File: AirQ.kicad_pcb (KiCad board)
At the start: 2 copper layers, 4 parts, among them U1 ESP32-H2-MINI-1-H2, U2 AP2112K-3.3, U3 AP2112K-1.8

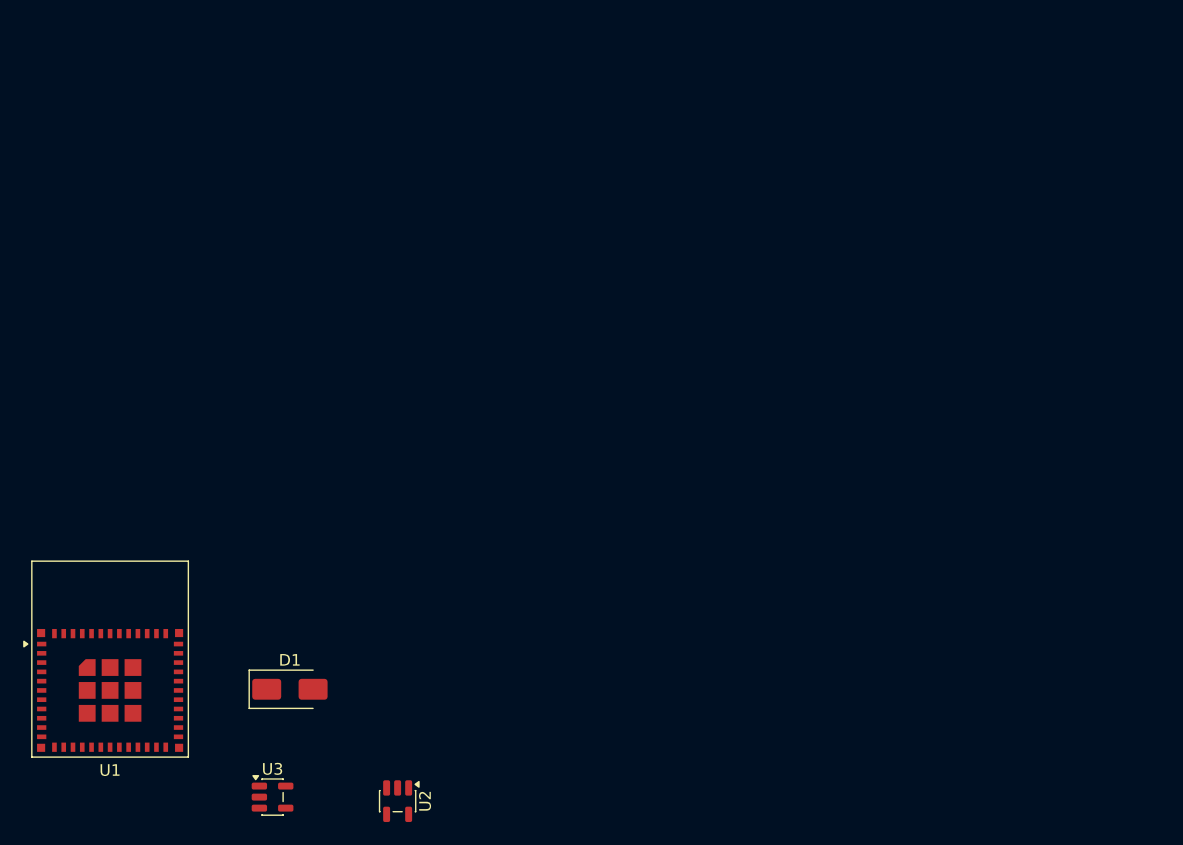
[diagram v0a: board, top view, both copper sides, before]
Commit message: Avances Viernes
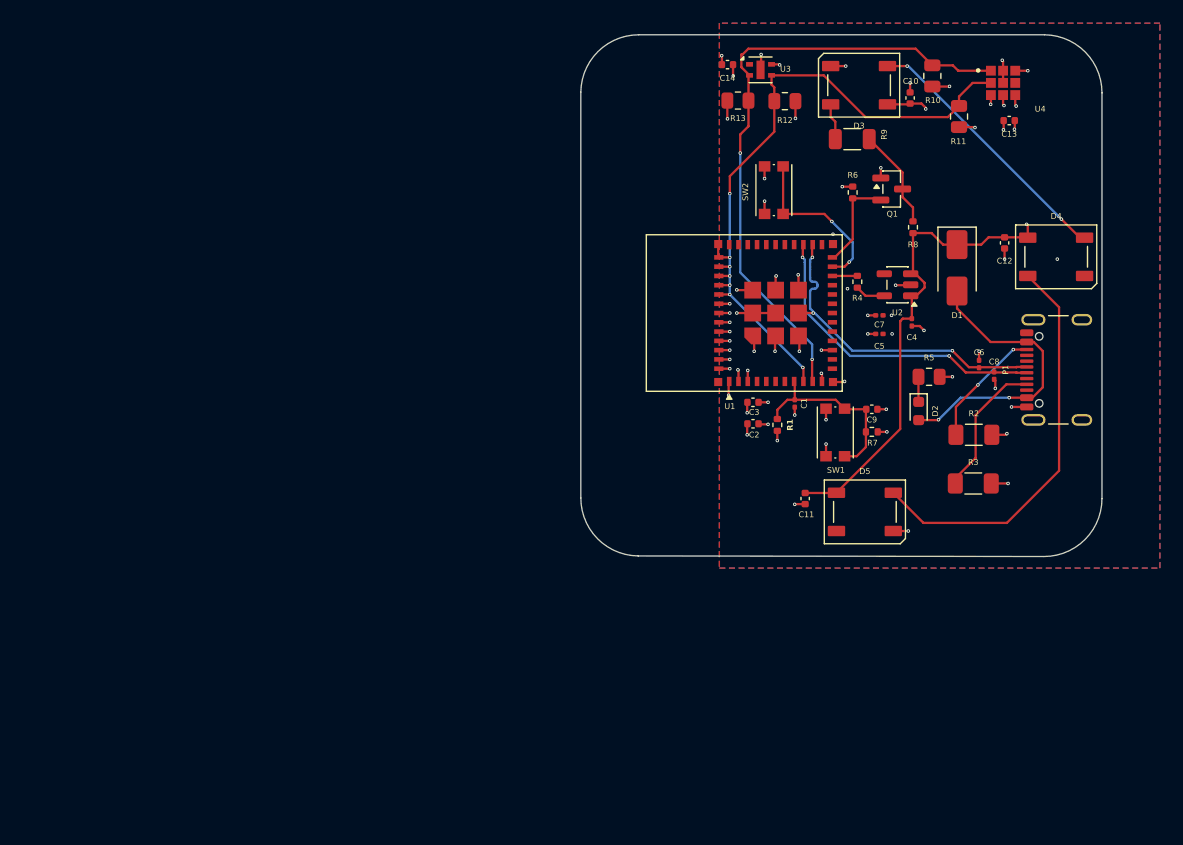
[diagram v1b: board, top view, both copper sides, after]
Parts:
- added C1: 1uF, Capacitor_SMD:C_0201_0603Metric, F.Cu at (173.5, 81.8)
- added C10: 0.1uF, Capacitor_SMD:C_0402_1005Metric, F.Cu at (183.4, 55.5)
- added C11: 0.1uF, Capacitor_SMD:C_0402_1005Metric, F.Cu at (174.4, 90.0)
- added C12: 0.1uF, Capacitor_SMD:C_0402_1005Metric, F.Cu at (191.6, 68.0)
- added C13: 10uF, Capacitor_SMD:C_0402_1005Metric, F.Cu at (192.0, 57.4)
- added C14: 0.1uF, Capacitor_SMD:C_0402_1005Metric, F.Cu at (167.7, 52.6)
- added C2: 10uF, Capacitor_SMD:C_0402_1005Metric, F.Cu at (169.9, 83.5)
- added C3: 0.1uF, Capacitor_SMD:C_0402_1005Metric, F.Cu at (169.9, 81.7)
- added C4: 1uF, Capacitor_SMD:C_0201_0603Metric, F.Cu at (183.6, 74.8)
- added C5: 1uF, Capacitor_SMD:C_0201_0603Metric, F.Cu at (180.8, 75.8)
- added C6: 1uF, Capacitor_SMD:C_0201_0603Metric, F.Cu at (189.4, 78.4)
- added C7: 1uF, Capacitor_SMD:C_0201_0603Metric, F.Cu at (180.8, 74.2)
- added C8: 1uF, Capacitor_SMD:C_0201_0603Metric, F.Cu at (190.7, 79.4)
- added C9: 0.1uF, Capacitor_SMD:C_0402_1005Metric, F.Cu at (180.2, 82.3)
- added D2: LED, LED_SMD:LED_0603_1608Metric, F.Cu at (184.2, 82.5)
- added D3: WS2812B, LED_SMD:LED_WS2812B_PLCC4_5.0x5.0mm_P3.2mm, F.Cu at (179.1, 54.4)
- added D4: WS2812B, LED_SMD:LED_WS2812B_PLCC4_5.0x5.0mm_P3.2mm, F.Cu at (196.1, 69.2)
- added D5: WS2812B, LED_SMD:LED_WS2812B_PLCC4_5.0x5.0mm_P3.2mm, F.Cu at (179.6, 91.2)
- added P1: USB_C_Plug_USB2.0, Connector_USB:USB_C_Receptacle_GCT_USB4105-xx-A_16P_TopMnt_Horizontal, F.Cu at (197.2, 78.9)
- added Q1: BSS138, Package_TO_SOT_SMD:SOT-23, F.Cu at (181.9, 63.3)
- added R1: 10K, Resistor_SMD:R_0402_1005Metric, F.Cu at (172.0, 83.7)
- added R10: 4.7K, Resistor_SMD:R_0805_2012Metric, F.Cu at (185.4, 53.5)
- added R11: 4.7K, Resistor_SMD:R_0805_2012Metric, F.Cu at (187.7, 57.0)
- added R12: 4.7K, Resistor_SMD:R_0805_2012Metric, F.Cu at (172.7, 55.7)
- added R13: 4.7K, Resistor_SMD:R_0805_2012Metric, F.Cu at (168.6, 55.7)
- added R2: 5.1K, Resistor_SMD:R_1206_3216Metric_Pad1.30x1.75mm_HandSolder, F.Cu at (188.9, 84.5)
- added R3: 5.1K, Resistor_SMD:R_1206_3216Metric_Pad1.30x1.75mm_HandSolder, F.Cu at (188.9, 88.7)
- added R4: 10K, Resistor_SMD:R_0402_1005Metric, F.Cu at (178.9, 71.3)
- added R5: 330, Resistor_SMD:R_0805_2012Metric, F.Cu at (185.1, 79.5)
- added R6: 10K, Resistor_SMD:R_0402_1005Metric, F.Cu at (178.5, 63.6)
- added R7: 10K, Resistor_SMD:R_0402_1005Metric, F.Cu at (180.2, 84.2)
- added R8: 10K, Resistor_SMD:R_0402_1005Metric, F.Cu at (183.7, 66.6)
- added R9: 470, Resistor_SMD:R_1206_3216Metric, F.Cu at (178.5, 59.0)
- added SW1: EN, Button_Switch_SMD:SW_Push_1P1T_NO_CK_KMR2, F.Cu at (177.0, 84.3)
- added SW2: EN, Button_Switch_SMD:SW_Push_1P1T_NO_CK_KMR2, F.Cu at (171.7, 63.4)
- added U4: ENS161-BLGM, ENS161:XDCR_ENS161-BLGM, F.Cu at (191.5, 54.1)
- U3: value AP2112K-1.8 -> ENS210; footprint Package_TO_SOT_SMD:SOT-23-5 -> Package_DFN_QFN:AMS_QFN-4-1EP_2x2mm_P0.95mm_EP0.7x1.6mm
- moved U3 75.5 mm to (170.6, 53.0)
- moved D1 68.1 mm to (187.5, 70.1), turned to -90 degrees
- moved U1 66.0 mm to (171.8, 74.0), turned to 90 degrees
- moved U2 62.0 mm to (182.4, 71.6), turned to 180 degrees
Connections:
- U1 pad 10: unconnected-(U1-IO01-Pad10) -> /SCL
- U1 pad 22: unconnected-(U1-IO08-Pad22) -> Net-(U1-IO08)
- U1 pad 23: unconnected-(U1-IO9-Pad23) -> /BOOT
- U1 pad 24: unconnected-(U1-IO22-Pad24) -> /LED_P
- U1 pad 25: D+ -> unconnected-(U1-IO25-Pad25)
- U1 pad 26: D- -> /D-
- U1 pad 27: unconnected-(U1-IO27-Pad27) -> /D+
- U1 pad 3: unconnected-(U1-3v3-Pad3) -> +3.3V
- U1 pad 49: unconnected-(U1-EPAD-Pad49) -> GND
- U1 pad 53: unconnected-(U1-GND-Pad53) -> GND
- U1 pad 8: unconnected-(U1-EN-Pad8) -> /RESET
- U1 pad 9: unconnected-(U1-IO0-Pad9) -> /SDA
- U3 pad 2: GND -> /SCL
- U3 pad 3: +3.3V -> /SDA
- U3 pad 4: unconnected-(U3-NC-Pad4) -> GND
- U3 pad 5: +1V8 -> GND
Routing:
- net GND: track 0.00 -> 60.8 mm, vias 0 -> 57
- net +5V: track 0.00 -> 58.8 mm, vias 0 -> 2
- net /SCL: track 0.00 -> 53.9 mm, vias 0 -> 2
- net /SDA: track 0.00 -> 52.8 mm, vias 0 -> 2
- net Net-(D4-DOUT): track 0.00 -> 35.2 mm
- net /D+: track 0.00 -> 27.1 mm, vias 0 -> 2
- net /D-: track 0.00 -> 27.1 mm, vias 0 -> 2
- net VBUS: track 0.00 -> 25.4 mm, vias 0 -> 2
- net Net-(D3-DOUT): track 0.00 -> 23.1 mm, vias 0 -> 2
- net +3.3V: track 0.00 -> 19.6 mm, vias 0 -> 19
- net /RESET: track 0.00 -> 16.2 mm
- net /BOOT: track 0.00 -> 14.6 mm, vias 0 -> 2
- net Net-(P1-CC): track 0.00 -> 12.1 mm
- net Net-(P1-VCONN): track 0.00 -> 10.6 mm, vias 0 -> 2
- net Net-(Q1-D): track 0.00 -> 8.65 mm
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- added copper zone on In2.Cu, net +3.3V
- added copper zone on B.Cu, net GND
- added copper zone on F.Cu, net GND
- added copper zone on In1.Cu, net GND
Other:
- board outline added: 44.9 x 45 mm
- copper layers 2 -> 4
